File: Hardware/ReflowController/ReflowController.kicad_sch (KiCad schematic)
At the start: 4 parts, among them J1 Conn_01x03_Socket

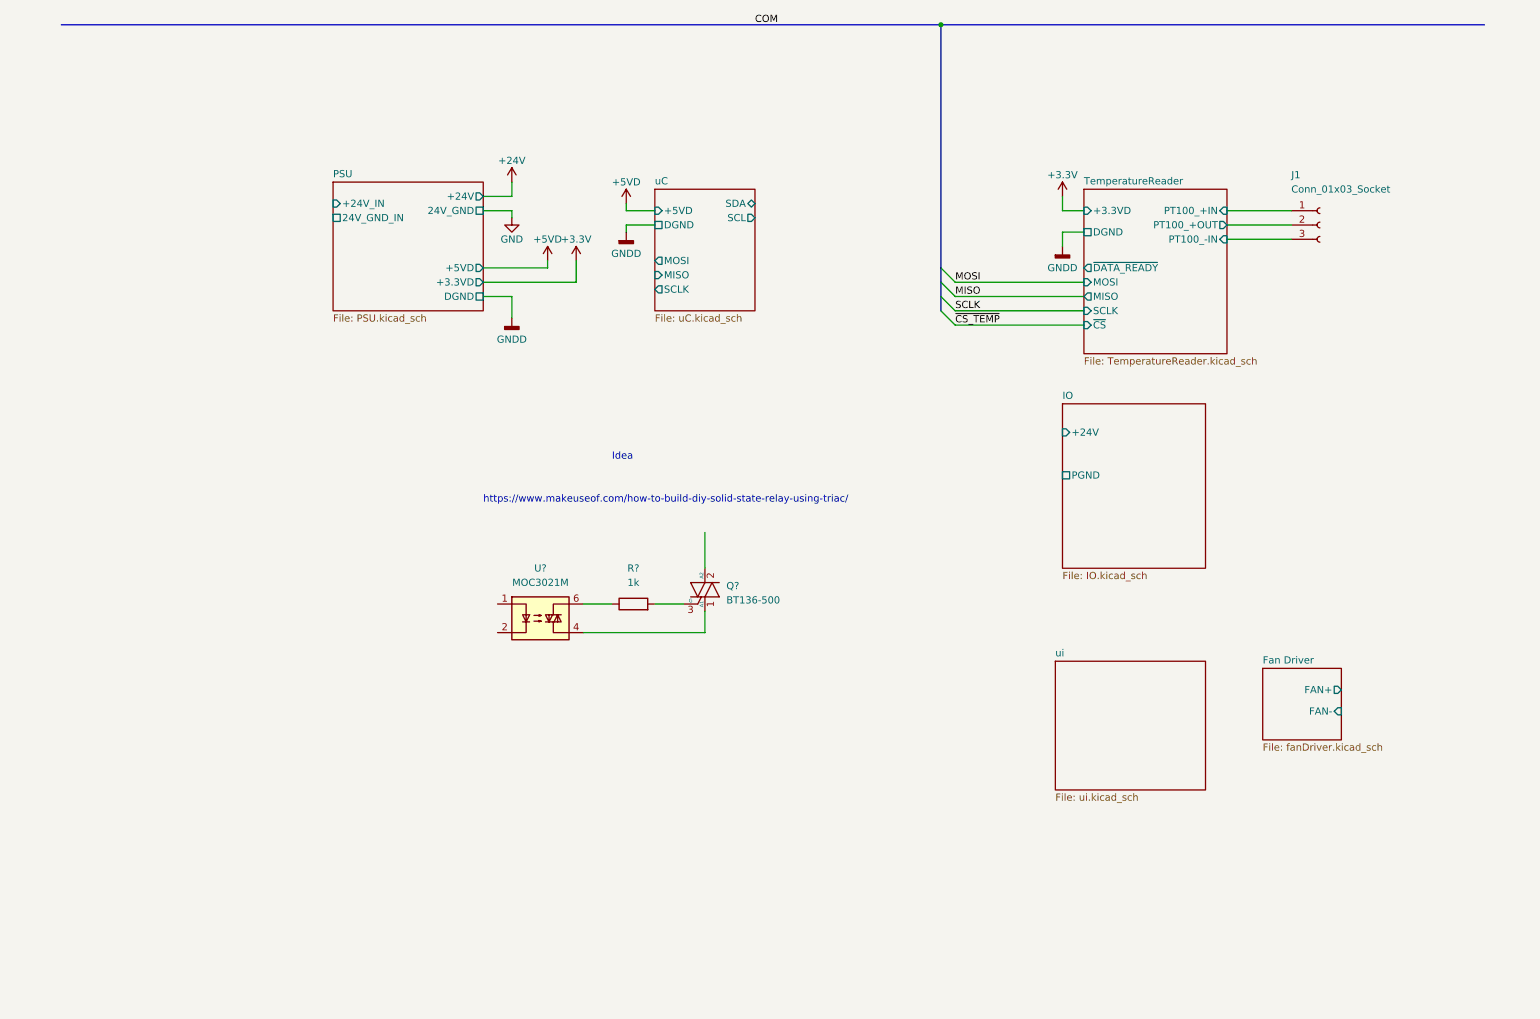
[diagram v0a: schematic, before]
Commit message: updated main schematic with kerem
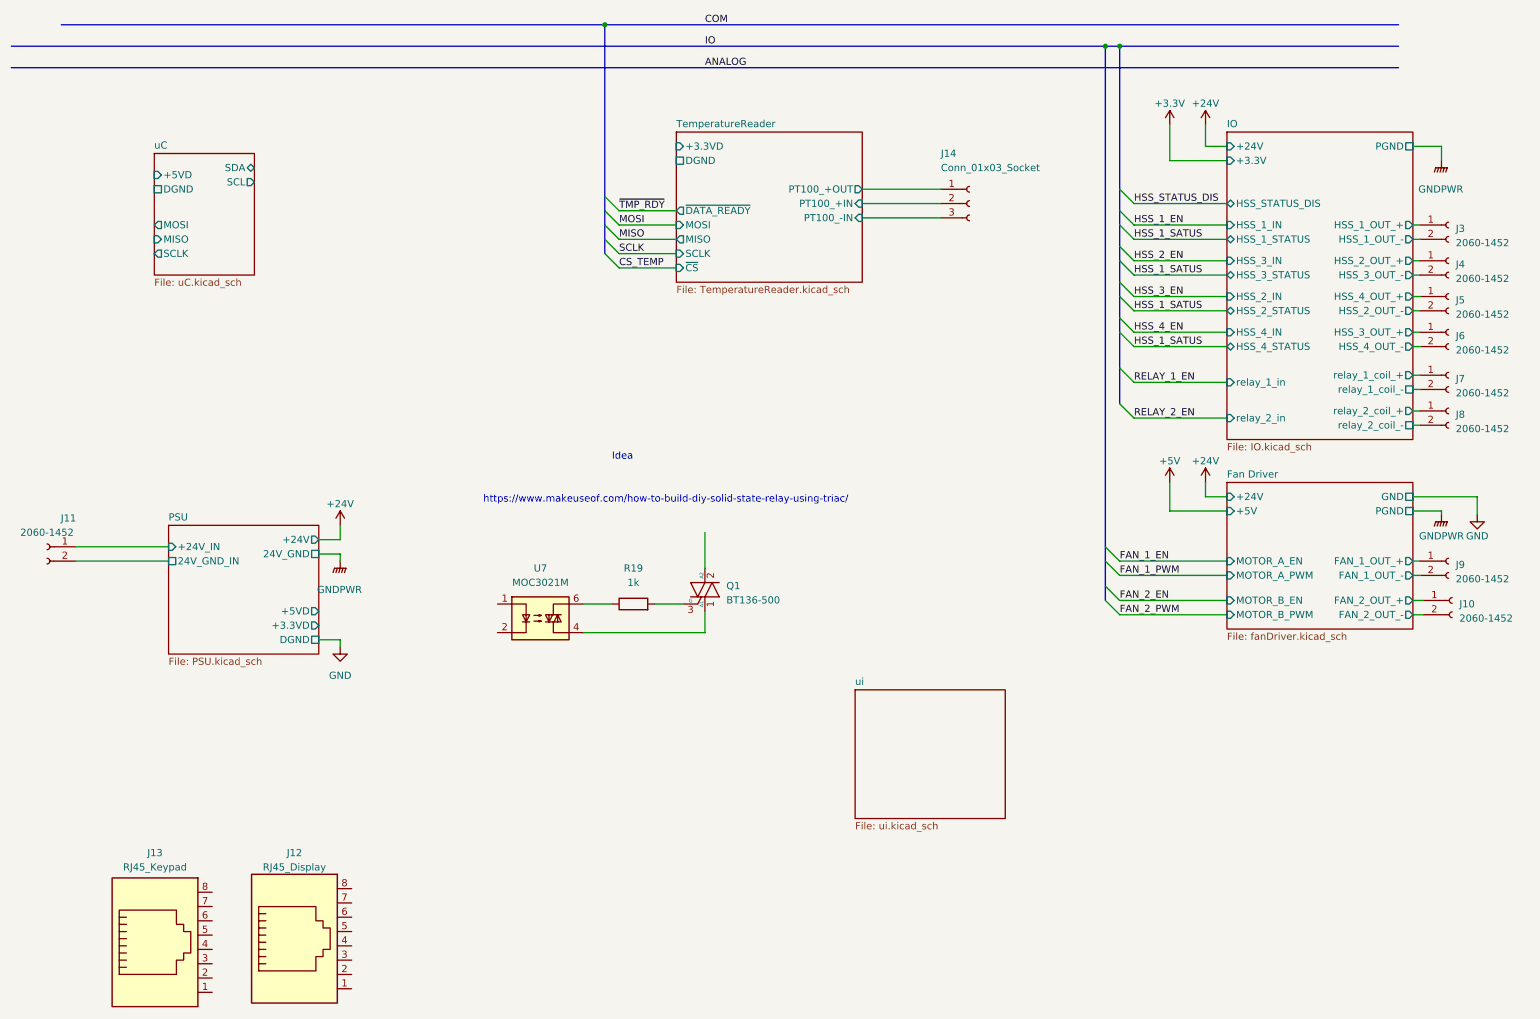
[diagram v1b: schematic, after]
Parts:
- removed J1: Conn_01x03_Socket, symbol Connector:Conn_01x03_Socket
- added J10, J11, J3, J4, J5, J6, J7, J8, J9: 2060-1452, 810_connectors_clable_to_Board:wago_2060-1452, symbol Connector:Conn_01x02_Socket
- added J12: RJ45_Display, Connector_RJ:RJ45_Amphenol_54602-x08_Horizontal, symbol Connector:RJ45
- added J13: RJ45_Keypad, Connector_RJ:RJ45_Amphenol_54602-x08_Horizontal, symbol Connector:RJ45
- added J14: Conn_01x03_Socket, 810_connectors_clable_to_Board:wago_2060-1453, symbol Connector:Conn_01x03_Socket
- gave numbers to parts that had none: 3
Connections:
- net PSU/+24V_IN: now also J11.1 (Pin_1)
- net PSU/24V_GND_IN: now also J11.2 (Pin_2)
- net TemperatureReader/PT100_+IN: now also J14.2 (Pin_2)
- net TemperatureReader/PT100_+OUT: now also J14.1 (Pin_1)
- net TemperatureReader/PT100_-IN: now also J14.3 (Pin_3)
- new net Fan Driver/FAN_1_OUT_+: J9.1 (Pin_1)
- new net Fan Driver/FAN_1_OUT_-: J9.2 (Pin_2)
- new net Fan Driver/FAN_2_OUT_+: J10.1 (Pin_1)
- new net Fan Driver/FAN_2_OUT_-: J10.2 (Pin_2)
- new net IO/HSS_1_OUT_+: J3.1 (Pin_1)
- new net IO/HSS_1_OUT_-: J3.2 (Pin_2)
- new net IO/HSS_2_OUT_+: J4.1 (Pin_1)
- new net IO/HSS_2_OUT_-: J5.2 (Pin_2)
- new net IO/HSS_3_OUT_+: J6.1 (Pin_1)
- new net IO/HSS_3_OUT_-: J4.2 (Pin_2)
- new net IO/HSS_4_OUT_+: J5.1 (Pin_1)
- new net IO/HSS_4_OUT_-: J6.2 (Pin_2)
- new net IO/relay_1_coil_+: J7.1 (Pin_1)
- new net IO/relay_1_coil_-: J7.2 (Pin_2)
- new net IO/relay_2_coil_+: J8.1 (Pin_1)
- new net IO/relay_2_coil_-: J8.2 (Pin_2)
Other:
- sheet Fan Driver ports: added +24V, +5V, FAN_1_OUT_+, FAN_1_OUT_-, FAN_2_OUT_+, FAN_2_OUT_-, GND, MOTOR_A_EN, MOTOR_A_PWM, MOTOR_B_EN, MOTOR_B_PWM, PGND; removed FAN+, FAN-
- sheet IO ports: added +3.3V, HSS_1_IN, HSS_1_OUT_+, HSS_1_OUT_-, HSS_1_STATUS, HSS_2_IN, HSS_2_OUT_+, HSS_2_OUT_-, HSS_2_STATUS, HSS_3_IN, HSS_3_OUT_+, HSS_3_OUT_-, HSS_3_STATUS, HSS_4_IN, HSS_4_OUT_+, HSS_4_OUT_-, HSS_4_STATUS, HSS_STATUS_DIS, relay_1_coil_+, relay_1_coil_-, relay_1_in, relay_2_coil_+, relay_2_coil_-, relay_2_in; removed none
- title: (none) -> Reflow Oven Control
